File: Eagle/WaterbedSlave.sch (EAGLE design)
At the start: 6 parts

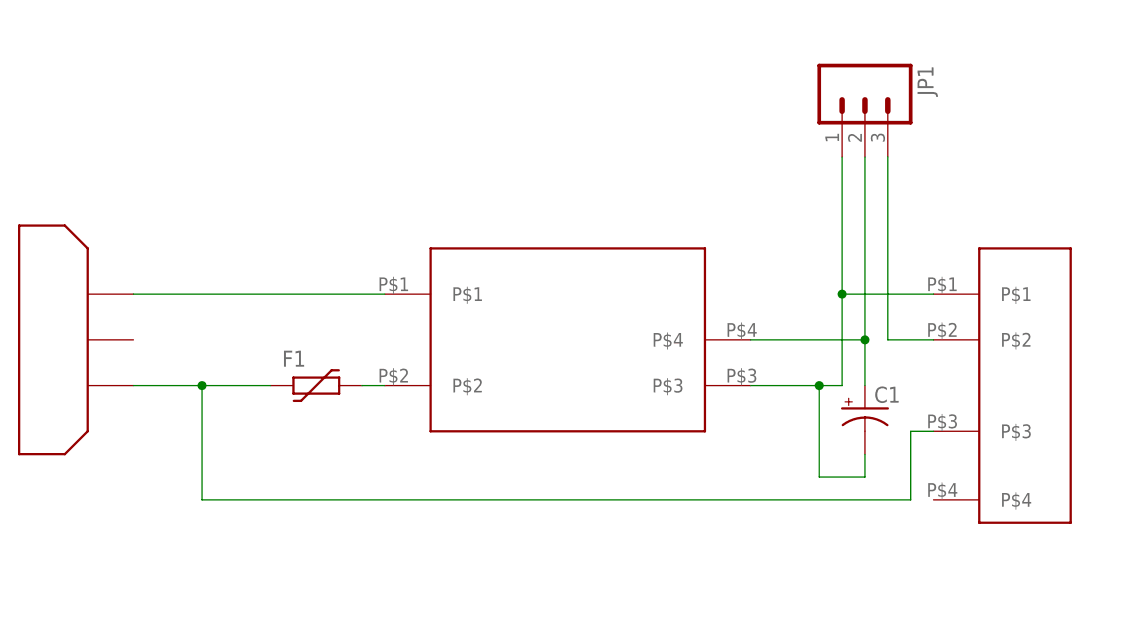
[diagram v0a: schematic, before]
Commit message: Update WaterbedSlave.sch
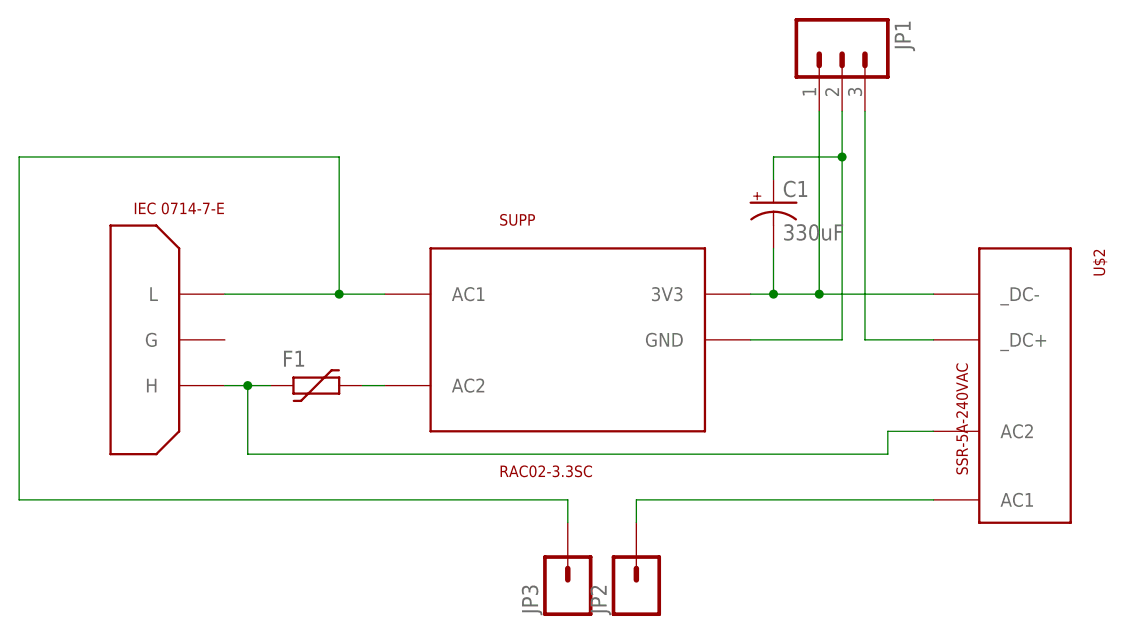
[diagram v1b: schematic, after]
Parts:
- removed U$1: RAC5A240VAC, CuriousTech:RAC5A240VAC
- added JP2, JP3: (no value), SparkFun-Connectors:M01PTH_2MM
- added SUPP: RAC02-3.3SC, CuriousTech:RAC02-3.3SC
- C1: value (none) -> 330uF
- U$3: value IEC -> IEC 0714-7-E
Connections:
- new net N$6: JP2.1, U$2.AC1
- net GND: now also SUPP.3V3, U$2._DC-; no longer U$1.P$3, U$2.P$1
- net N$1: now also JP3.1, SUPP.AC1; no longer U$1.P$1
- net N$12: now also SUPP.AC2; no longer U$1.P$2
- net N$14: now also U$2.AC2; no longer U$2.P$3
- net N$15: now also SUPP.GND; no longer U$1.P$4
- net N$16: now also U$2._DC+; no longer U$2.P$2
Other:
- moved on the sheet: C1, JP1
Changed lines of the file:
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@@
 </classes>
 <parts>
-<part name="U$1" library="CuriousTech" deviceset="RAC5A240VAC" device=""/>
 <part name="U$2" library="CuriousTech" deviceset="SSR-5A-240VAC" device=""/>
 <part name="JP1" library="SparkFun-Connectors" deviceset="M03" device="POLAR_LOCK"/>
 <part name="F1" library="dp_devices" deviceset="FUSE_PTC" device="-1812"/>
-<part name="C1" library="resistor" deviceset="CPOL-US" device="TT5D9"/>
-<part name="U$3" library="CuriousTech" deviceset="IEC" device=""/>
+<part name="C1" library="resistor" deviceset="CPOL-US" device="TT5D9" value="330uF"/>
+<part name="U$3" library="CuriousTech" deviceset="IEC" device="" value="IEC 0714-7-E"/>
+<part name="SUPP" library="CuriousTech" deviceset="RAC02-3.3SC" device=""/>
+<part name="JP3" library="SparkFun-Connectors" deviceset="M01" device="PTH_2MM"/>
+<part name="JP2" library="SparkFun-Connectors" deviceset="M01" device="PTH_2MM"/>
 </parts>
 <sheets>
@@
 </plain>
 <instances>
-<instance part="U$1" gate="G$1" x="60.96" y="60.96"/>
 <instance part="U$2" gate="G$1" x="111.76" y="55.88" rot="R270"/>
-<instance part="JP1" gate="G$1" x="93.98" y="88.9" rot="R270"/>
+<instance part="JP1" gate="G$1" x="91.44" y="93.98" rot="R270"/>
 <instance part="F1" gate="G$1" x="33.02" y="55.88"/>
-<instance part="C1" gate="G$1" x="93.98" y="53.34"/>
-<instance part="U$3" gate="G$1" x="7.62" y="60.96" rot="MR270"/>
+<instance part="C1" gate="G$1" x="83.82" y="76.2"/>
+<instance part="U$3" gate="G$1" x="17.78" y="55.88" rot="MR180"/>
+<instance part="SUPP" gate="G$1" x="60.96" y="60.96"/>
+<instance part="JP3" gate="G$1" x="60.96" y="33.02" rot="R90"/>
+<instance part="JP2" gate="G$1" x="68.58" y="33.02" rot="R90"/>
 </instances>
 <busses>
@@
 <net name="GND" class="0">
 <segment>
-<pinref part="U$1" gate="G$1" pin="P$3"/>
-<wire x1="81.28" y1="55.88" x2="88.9" y2="55.88" width="0.1524" layer="91"/>
 <pinref part="JP1" gate="G$1" pin="1"/>
-<pinref part="U$2" gate="G$1" pin="P$1"/>
-<wire x1="88.9" y1="55.88" x2="91.44" y2="55.88" width="0.1524" layer="91"/>
-<wire x1="91.44" y1="66.04" x2="91.44" y2="81.28" width="0.1524" layer="91"/>
-<wire x1="101.6" y1="66.04" x2="91.44" y2="66.04" width="0.1524" layer="91"/>
-<wire x1="91.44" y1="66.04" x2="91.44" y2="55.88" width="0.1524" layer="91"/>
-<junction x="91.44" y="66.04"/>
-<wire x1="88.9" y1="55.88" x2="88.9" y2="45.72" width="0.1524" layer="91"/>
-<wire x1="88.9" y1="45.72" x2="93.98" y2="45.72" width="0.1524" layer="91"/>
-<wire x1="93.98" y1="45.72" x2="93.98" y2="48.26" width="0.1524" layer="91"/>
-<junction x="88.9" y="55.88"/>
+<pinref part="U$2" gate="G$1" pin="_DC-"/>
+<wire x1="88.9" y1="66.04" x2="88.9" y2="86.36" width="0.1524" layer="91"/>
+<wire x1="101.6" y1="66.04" x2="88.9" y2="66.04" width="0.1524" layer="91"/>
+<junction x="88.9" y="66.04"/>
 <pinref part="C1" gate="G$1" pin="-"/>
+<wire x1="83.82" y1="66.04" x2="83.82" y2="71.12" width="0.1524" layer="91"/>
+<wire x1="81.28" y1="66.04" x2="83.82" y2="66.04" width="0.1524" layer="91"/>
+<wire x1="83.82" y1="66.04" x2="88.9" y2="66.04" width="0.1524" layer="91"/>
+<junction x="83.82" y="66.04"/>
+<pinref part="SUPP" gate="G$1" pin="3V3"/>
 </segment>
 </net>
 <net name="N$15" class="0">
 <segment>
-<pinref part="U$1" gate="G$1" pin="P$4"/>
-<wire x1="81.28" y1="60.96" x2="93.98" y2="60.96" width="0.1524" layer="91"/>
+<wire x1="81.28" y1="60.96" x2="91.44" y2="60.96" width="0.1524" layer="91"/>
 <pinref part="JP1" gate="G$1" pin="2"/>
-<wire x1="93.98" y1="60.96" x2="93.98" y2="81.28" width="0.1524" layer="91"/>
-<wire x1="93.98" y1="60.96" x2="93.98" y2="55.88" width="0.1524" layer="91"/>
-<junction x="93.98" y="60.96"/>
+<wire x1="91.44" y1="60.96" x2="91.44" y2="81.28" width="0.1524" layer="91"/>
+<pinref part="SUPP" gate="G$1" pin="GND"/>
 <pinref part="C1" gate="G$1" pin="+"/>
+<wire x1="91.44" y1="81.28" x2="91.44" y2="86.36" width="0.1524" layer="91"/>
+<wire x1="83.82" y1="78.74" x2="83.82" y2="81.28" width="0.1524" layer="91"/>
+<wire x1="83.82" y1="81.28" x2="91.44" y2="81.28" width="0.1524" layer="91"/>
+<junction x="91.44" y="81.28"/>
 </segment>
 </net>
@@
 <segment>
 <pinref part="JP1" gate="G$1" pin="3"/>
-<wire x1="96.52" y1="81.28" x2="96.52" y2="60.96" width="0.1524" layer="91"/>
-<pinref part="U$2" gate="G$1" pin="P$2"/>
-<wire x1="96.52" y1="60.96" x2="101.6" y2="60.96" width="0.1524" layer="91"/>
+<wire x1="93.98" y1="86.36" x2="93.98" y2="60.96" width="0.1524" layer="91"/>
+<pinref part="U$2" gate="G$1" pin="_DC+"/>
+<wire x1="93.98" y1="60.96" x2="101.6" y2="60.96" width="0.1524" layer="91"/>
 </segment>
 </net>
@@
 <segment>
 <pinref part="F1" gate="G$1" pin="1"/>
-<wire x1="27.94" y1="55.88" x2="20.32" y2="55.88" width="0.1524" layer="91"/>
-<wire x1="20.32" y1="55.88" x2="20.32" y2="43.18" width="0.1524" layer="91"/>
-<wire x1="20.32" y1="43.18" x2="99.06" y2="43.18" width="0.1524" layer="91"/>
-<wire x1="99.06" y1="43.18" x2="99.06" y2="50.8" width="0.1524" layer="91"/>
-<pinref part="U$2" gate="G$1" pin="P$3"/>
-<wire x1="99.06" y1="50.8" x2="101.6" y2="50.8" width="0.1524" layer="91"/>
+<wire x1="27.94" y1="55.88" x2="25.4" y2="55.88" width="0.1524" layer="91"/>
+<wire x1="25.4" y1="55.88" x2="25.4" y2="48.26" width="0.1524" layer="91"/>
+<wire x1="25.4" y1="48.26" x2="96.52" y2="48.26" width="0.1524" layer="91"/>
+<wire x1="96.52" y1="48.26" x2="96.52" y2="50.8" width="0.1524" layer="91"/>
+<pinref part="U$2" gate="G$1" pin="AC2"/>
+<wire x1="96.52" y1="50.8" x2="101.6" y2="50.8" width="0.1524" layer="91"/>
 <pinref part="U$3" gate="G$1" pin="H"/>
-<wire x1="12.7" y1="55.88" x2="20.32" y2="55.88" width="0.1524" layer="91"/>
-<junction x="20.32" y="55.88"/>
+<wire x1="22.86" y1="55.88" x2="25.4" y2="55.88" width="0.1524" layer="91"/>
+<junction x="25.4" y="55.88"/>
 </segment>
 </net>
@@
 <segment>
 <pinref part="F1" gate="G$1" pin="2"/>
-<pinref part="U$1" gate="G$1" pin="P$2"/>
 <wire x1="38.1" y1="55.88" x2="40.64" y2="55.88" width="0.1524" layer="91"/>
+<pinref part="SUPP" gate="G$1" pin="AC2"/>
 </segment>
 </net>
@@
 <segment>
 <pinref part="U$3" gate="G$1" pin="L"/>
-<pinref part="U$1" gate="G$1" pin="P$1"/>
-<wire x1="12.7" y1="66.04" x2="40.64" y2="66.04" width="0.1524" layer="91"/>
+<wire x1="22.86" y1="66.04" x2="35.56" y2="66.04" width="0.1524" layer="91"/>
+<pinref part="SUPP" gate="G$1" pin="AC1"/>
+<wire x1="35.56" y1="66.04" x2="40.64" y2="66.04" width="0.1524" layer="91"/>
+<wire x1="60.96" y1="40.64" x2="60.96" y2="43.18" width="0.1524" layer="91"/>
+<wire x1="60.96" y1="43.18" x2="0" y2="43.18" width="0.1524" layer="91"/>
+<wire x1="0" y1="43.18" x2="0" y2="81.28" width="0.1524" layer="91"/>
+<wire x1="0" y1="81.28" x2="35.56" y2="81.28" width="0.1524" layer="91"/>
+<wire x1="35.56" y1="81.28" x2="35.56" y2="66.04" width="0.1524" layer="91"/>
+<junction x="35.56" y="66.04"/>
+<pinref part="JP3" gate="G$1" pin="1"/>
 </segment>
 </net>
+<net name="N$6" class="0">
+<segment>
+<pinref part="U$2" gate="G$1" pin="AC1"/>
+<wire x1="101.6" y1="43.18" x2="68.58" y2="43.18" width="0.1524" layer="91"/>
+<wire x1="68.58" y1="43.18" x2="68.58" y2="40.64" width="0.1524" layer="91"/>
+<pinref part="JP2" gate="G$1" pin="1"/>
+</segment>
+</net>
